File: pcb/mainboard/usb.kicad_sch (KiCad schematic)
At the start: 30 parts, among them J601 USB_A, J602 USB_A, J603 USB_C_Receptacle_USB2.0, U601 USB2514B_Bi, U602 AP2171W, U603 AP2171W, U604 FUSB302BMPX, U605 USBLC6-2P6, Y601 24MHz

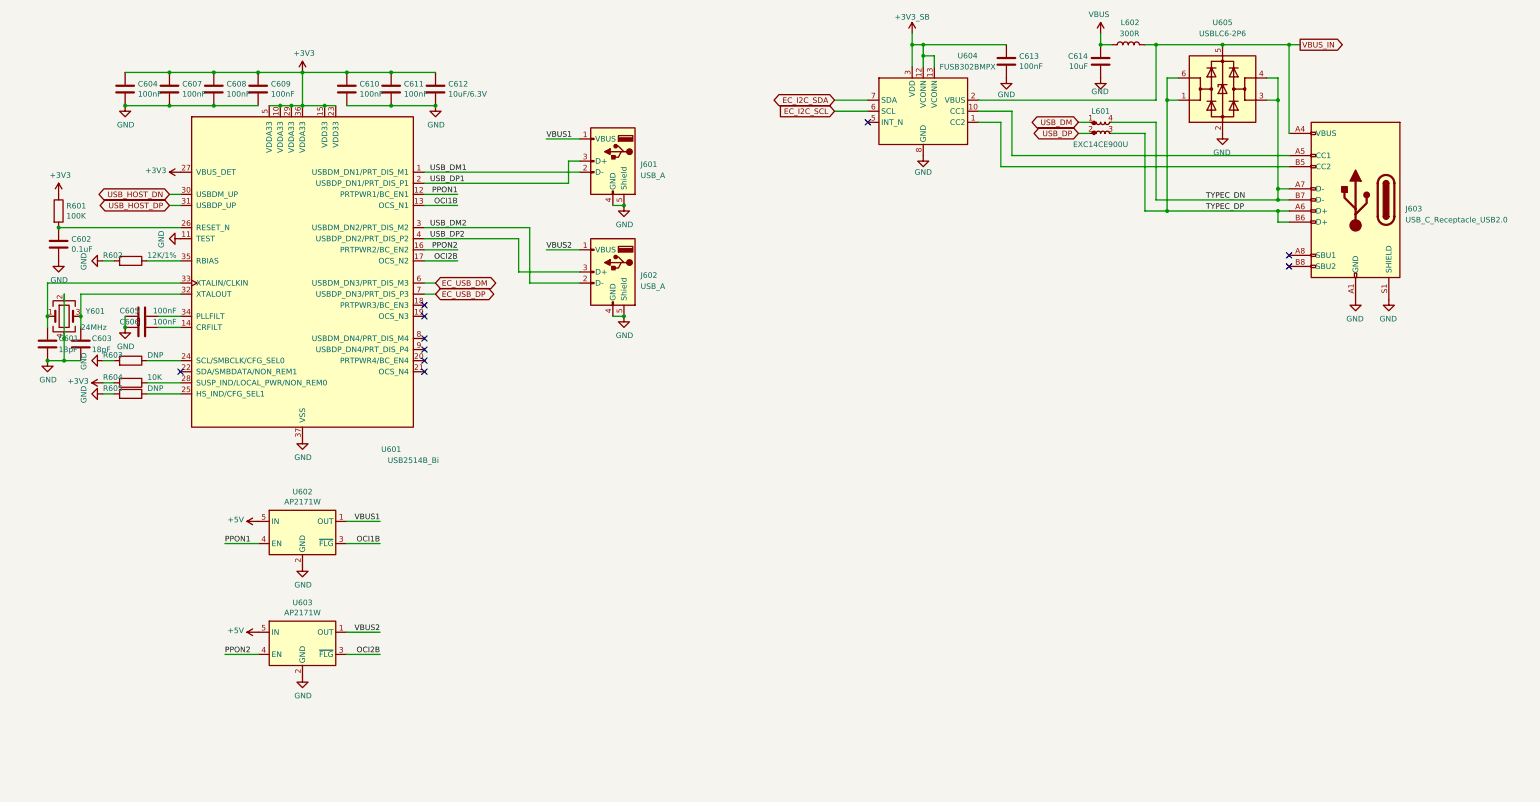
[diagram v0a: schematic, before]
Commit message: - pcb: start r0p1 layout
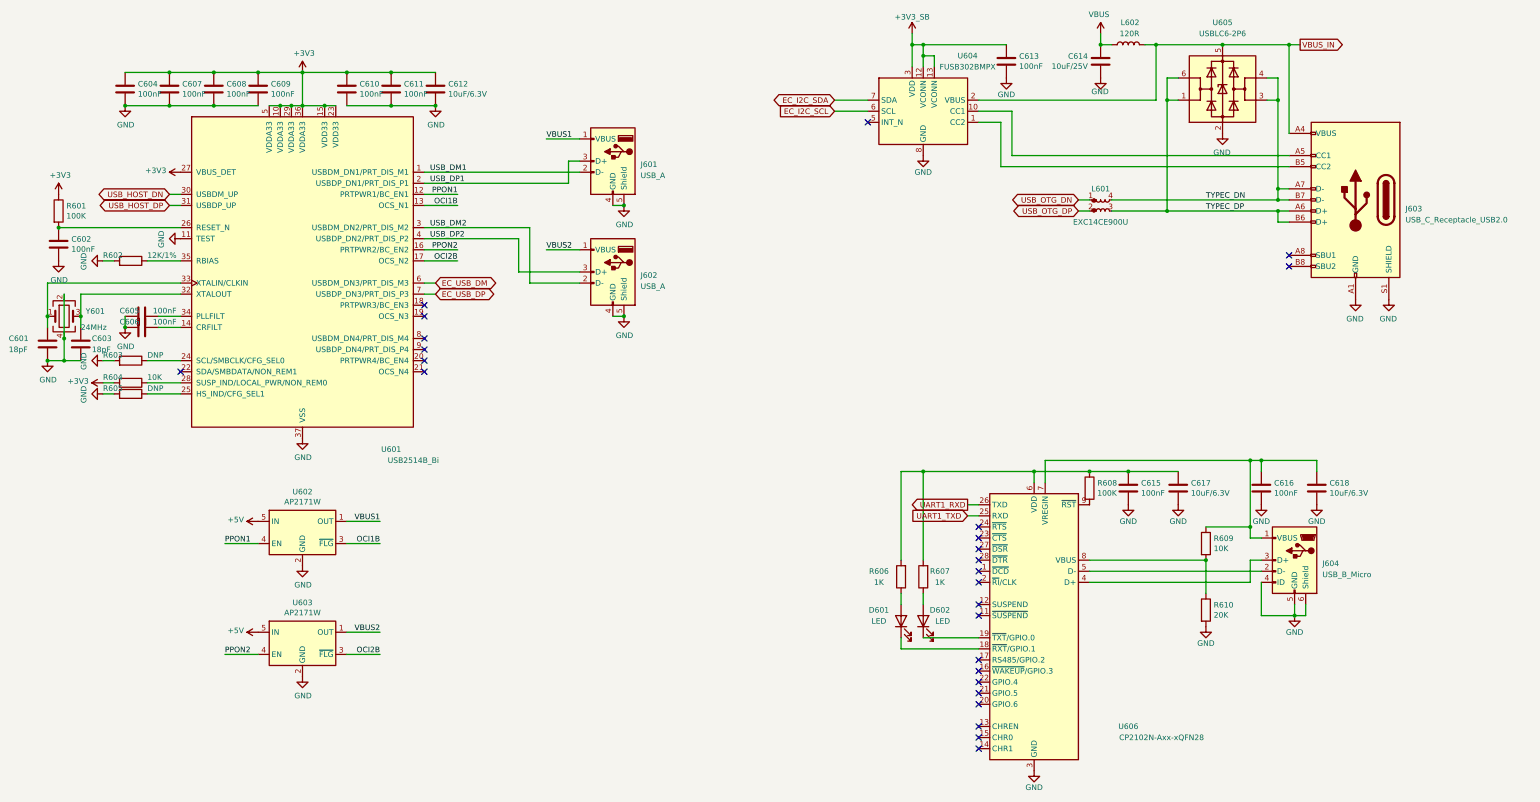
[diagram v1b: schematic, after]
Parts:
- added C615, C616: 100nF, Capacitor_SMD:C_0402_1005Metric, symbol Device:C
- added C617, C618: 10uF/6.3V, Capacitor_SMD:C_0603_1608Metric, symbol Device:C
- added D601, D602: LED, LED_SMD:LED_0603_1608Metric, symbol Device:LED
- added J604: USB_B_Micro, Connector_USB:USB_Micro-B_Amphenol_10103594-0001LF_Horizontal, symbol Connector:USB_B_Micro
- added R606, R607: 1K, Resistor_SMD:R_0402_1005Metric, symbol Device:R
- added R608: 100K, Resistor_SMD:R_0402_1005Metric, symbol Device:R
- added R609: 10K, Resistor_SMD:R_0402_1005Metric, symbol Device:R
- added R610: 20K, Resistor_SMD:R_0402_1005Metric, symbol Device:R
- added U606: CP2102N-Axx-xQFN28, Package_DFN_QFN:QFN-28-1EP_5x5mm_P0.5mm_EP3.35x3.35mm, symbol Interface_USB:CP2102N-Axx-xQFN28
- C602: value 0.1uF -> 100nF; footprint (none) -> Capacitor_SMD:C_0402_1005Metric
- C604, C607, C608, C609, C610, C611: footprint (none) -> Capacitor_SMD:C_0402_1005Metric
- C612: footprint (none) -> Capacitor_SMD:C_0603_1608Metric
- C613: footprint Capacitor_SMD:C_0201_0603Metric -> Capacitor_SMD:C_0402_1005Metric
- C614: value 10uF -> 10uF/25V; footprint Capacitor_SMD:C_0402_1005Metric -> Capacitor_SMD:C_0805_2012Metric
- J601, J602: footprint Connector_USB:USB_A_Molex_67643_Horizontal -> footprints:Connector_USB_905-562A2021S10100
- L601: footprint footprint:L_CommonModeChoke_Panasonic_EXC14CE -> footprints:L_CommonModeChoke_Panasonic_EXC14CE
- L602: value 300R -> 120R
- R601: footprint (none) -> Resistor_SMD:R_0402_1005Metric
- R602, R603, R604, R605: footprint Resistor_SMD:R_0603_1608Metric -> Resistor_SMD:R_0402_1005Metric
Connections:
- net GND: now also C615.2, C616.2, C617.2, C618.2, J604.4 (ID), J604.5 (GND), J604.6 (Shield), R610.2, U606.29 (GND), U606.3 (GND)
- net USB_DM renamed USB_OTG_DN
- net USB_DP renamed USB_OTG_DP
- new net: D601.2 (A), R606.1
- new net: C615.1, C617.1, R606.2, R607.2, R608.1, U606.6 (VDD)
- new net: D601.1 (K), U606.18 (~RXT~/GPIO.1)
- new net: D602.1 (K), U606.19 (~TXT~/GPIO.0)
- new net: J604.3 (D+), U606.4 (D+)
- new net: J604.2 (D-), U606.5 (D-)
- new net: C616.1, C618.1, J604.1 (VBUS), R609.1, U606.7 (VREGIN)
- new net: R609.2, R610.1, U606.8 (VBUS)
- new net: R608.2, U606.9 (~RST)
- new net: D602.2 (A), R607.1
- new net UART1_RXD: U606.26 (TXD)
- new net UART1_TXD: U606.25 (RXD)
- no-connect marks 10 -> 26
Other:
- company: Copyright EI-2030 2021. -> Copyright EI-2030 2021. / Engineer: Wenting Zhang
- title: Archer -> Archer Mainboard
- moved on the sheet: L601
